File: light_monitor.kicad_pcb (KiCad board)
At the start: 2 copper layers, 50.2 x 50.2 mm, 21 parts, among them IC1 TSL237S-LF, J1 Conn_01x03, J2 Conn_01x04_Male, U1 STM32L432KCUx, U2 STDC14, U3 TG-3541CE

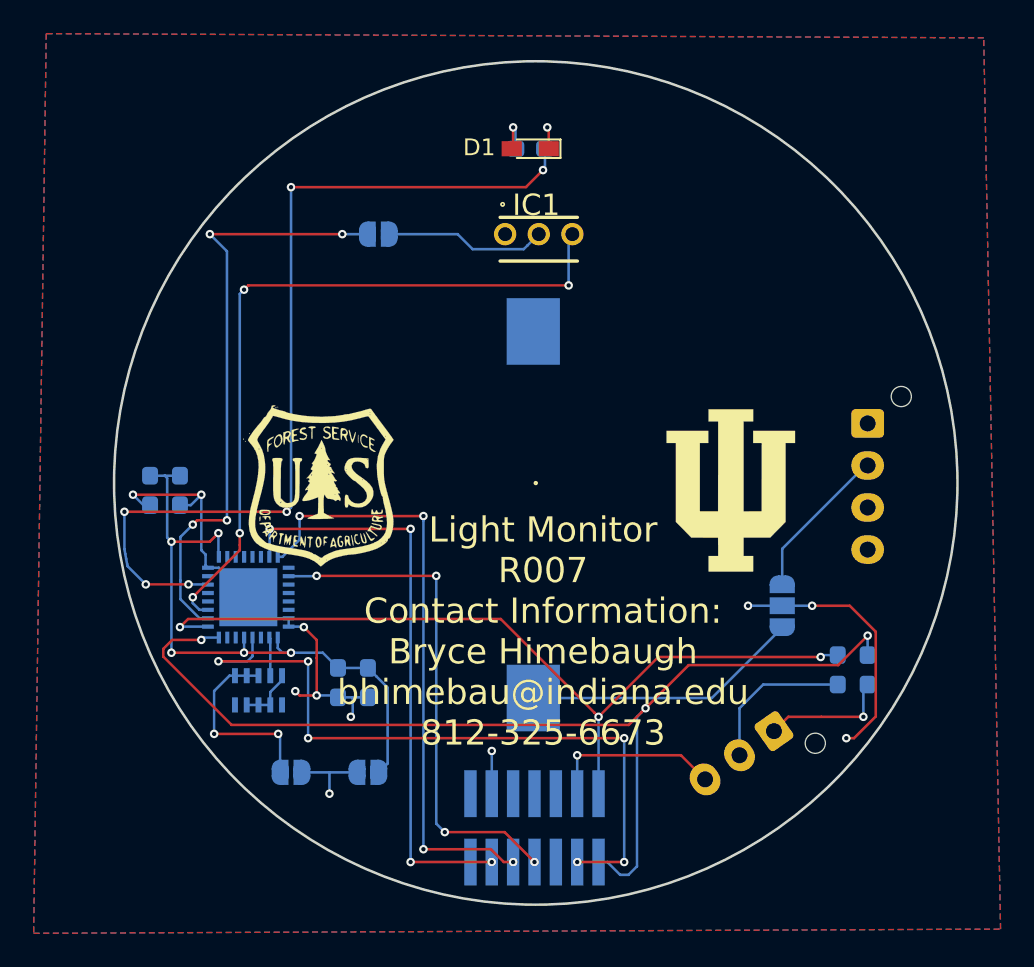
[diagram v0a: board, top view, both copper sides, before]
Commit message: revision 8 sent to fab
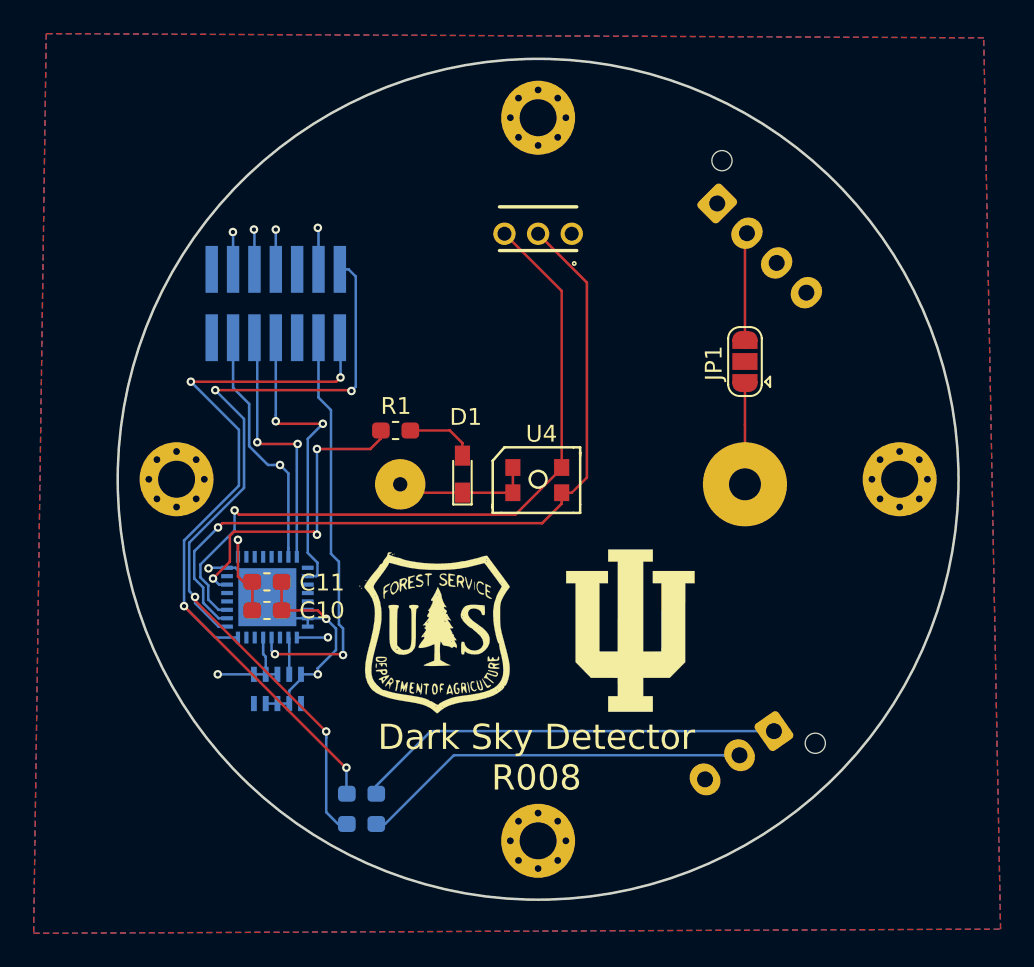
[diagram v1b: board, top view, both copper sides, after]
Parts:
- removed C8: 2.2uF, Capacitor_SMD:C_0603_1608Metric_Pad1.05x0.95mm_HandSolder
- removed C9: 0.1uF, Capacitor_SMD:C_0603_1608Metric_Pad1.05x0.95mm_HandSolder
- removed IC1: TSL237S-LF, SamacSys_Parts_3:TSL237S-LF
- removed JP2, JP3, JP4: Jumper_2_Open, Jumper:SolderJumper-2_P1.3mm_Open_RoundedPad1.0x1.5mm
- added H1: MountingHole, MountingHole:MountingHole_2.2mm_M2_Pad_Via, F.Cu at (113.5, 83.5)
- added H2: MountingHole, MountingHole:MountingHole_2.2mm_M2_Pad_Via, F.Cu at (135.0, 105.0)
- added H3: MountingHole, MountingHole:MountingHole_2.2mm_M2_Pad_Via, F.Cu at (113.5, 126.5)
- added H4: MountingHole, MountingHole:MountingHole_2.2mm_M2_Pad_Via, F.Cu at (92.0, 105.0)
- added U4: sm_tsl237, bhimebau_lightsensor:tsl237t, F.Cu at (114.1, 102.2)
- added e: TSL237S-LF, SamacSys_Parts_3:TSL237S-LF, F.Cu at (113.5, 90.4)
- BT1: footprint bhimebau_battery:Keystone_1091TR -> bhimebau_battery:BR2330A_Horizontal_Circular_Holes
- C10, C11, JP1: moved to F.Cu
- R1: value 300 -> 4.7k; moved to F.Cu
- moved U2 34.8 mm to (97.9, 94.5)
- moved R3 31.0 mm to (103.0, 123.7), turned to 0 degrees
- moved R4 29.8 mm to (103.0, 125.5), turned to 0 degrees
- moved D1 19.8 mm to (109.0, 104.7), turned to 90 degrees
- moved R1 18.6 mm to (105.0, 102.1), turned to 0 degrees
- moved J2 15.8 mm to (124.2, 88.6), turned to 315 degrees
- moved JP1 14.7 mm to (125.8, 98.0)
- moved G*** 11.1 mm to (107.5, 114.2)
- moved G*** 10.3 mm to (119.0, 114.0)
- moved C10 9.96 mm to (97.4, 112.8), turned to 0 degrees
- moved C11 7.50 mm to (97.4, 111.1), turned to 0 degrees
- moved BT1 2.96 mm to (115.5, 105.3), turned to 90 degrees
- moved U1 1.13 mm to (97.4, 112.0)
- moved U3 1.13 mm to (94.6, 119.3)
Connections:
- C10 pad 1: /l432_pwr -> VDD
- C11 pad 1: /l432_pwr -> VDD
- U1 pad 1: /l432_pwr -> VDD
- U1 pad 17: /l432_pwr -> VDD
- U1 pad 5: /l432_pwr -> VDD
- U3 pad 1: Net-(JP2-Pad2) -> VDD
- U3 pad 2: Net-(JP2-Pad2) -> VDD
- U3 pad 3: Net-(JP2-Pad2) -> VDD
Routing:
- net /l432_pwr: track 38.3 -> 0.00 mm, vias 5 -> 0
- net Net-(R1-Pad1): track 54.3 -> 18.9 mm, vias 6 -> 3
- net /SWDCLK: track 36.0 -> 15.5 mm, vias 4 -> 2
- net /SWDIO: track 34.7 -> 15.0 mm, vias 4 -> 1
- net /TX: track 64.4 -> 46.4 mm, vias 3 -> 4
- net Net-(J1-Pad1): track 7.70 -> 25.5 mm, vias 1 -> 0
- net /NRST: track 42.1 -> 24.6 mm, vias 6 -> 2
- net Net-(J1-Pad2): track 9.22 -> 23.3 mm
- net /SWO: track 30.3 -> 18.0 mm, vias 4 -> 2
- net Net-(JP2-Pad2): track 11.7 -> 0.00 mm, vias 2 -> 0
- net Net-(BT1-Pad1): track 16.5 -> 6.00 mm
- net /tsl237_pwr: track 35.8 -> 46.3 mm, vias 4 -> 1
- net Net-(IC1-Pad2): track 9.63 -> 0.00 mm
- net VDD: track 22.6 -> 15.7 mm, vias 5 -> 4
- net Net-(J2-Pad2): track 9.22 -> 6.38 mm
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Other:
- board size 50.2 x 50.2 mm -> 50 x 50 mm
- board text added: "Dark Sky Detector R008"
- board text removed: "Light Monitor R007 Contact Information: Bryce Himebaugh bhimebau@indiana.edu 812-325-6673"
- board text removed: "batt"
- board text removed: "board"
- board text removed: "mon"
